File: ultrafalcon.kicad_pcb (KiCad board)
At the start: 2 copper layers, 66.3 x 66.3 mm, 1 part, among them SW1 RotaryEncoder

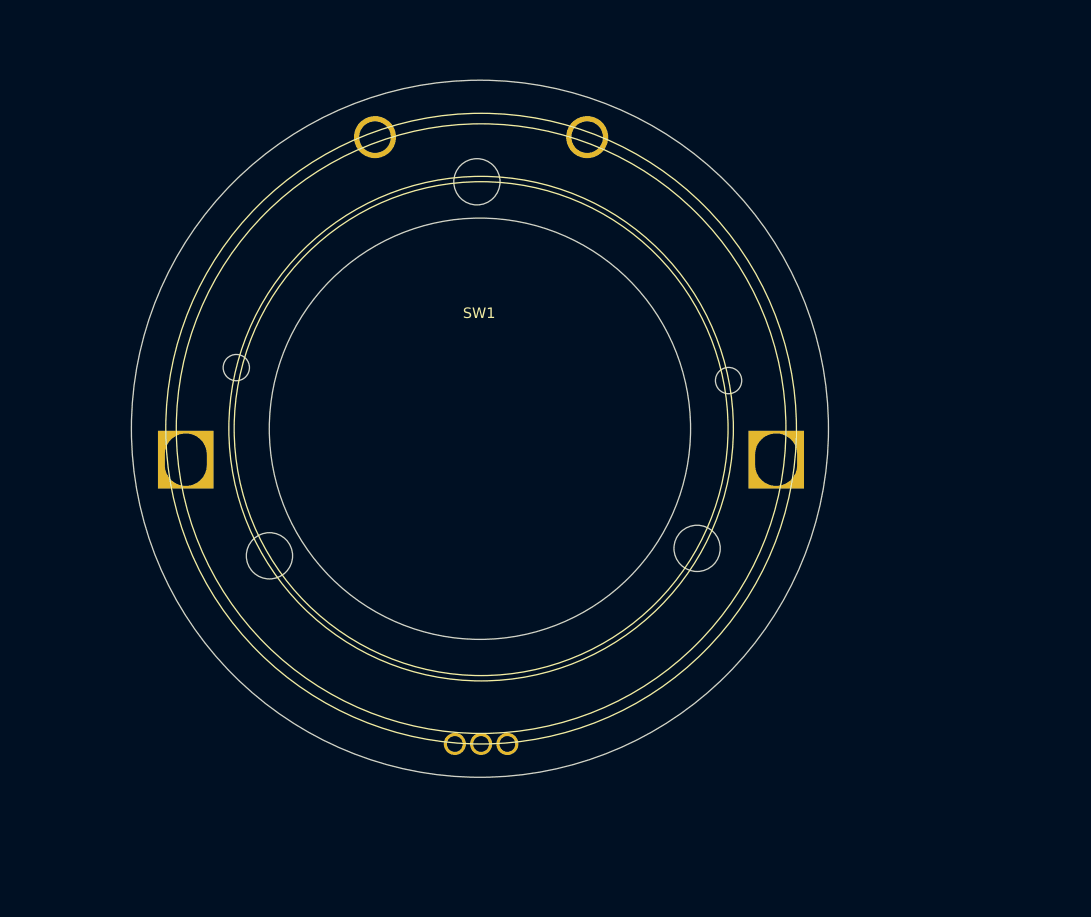
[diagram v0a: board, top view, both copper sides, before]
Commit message: jan17 updates
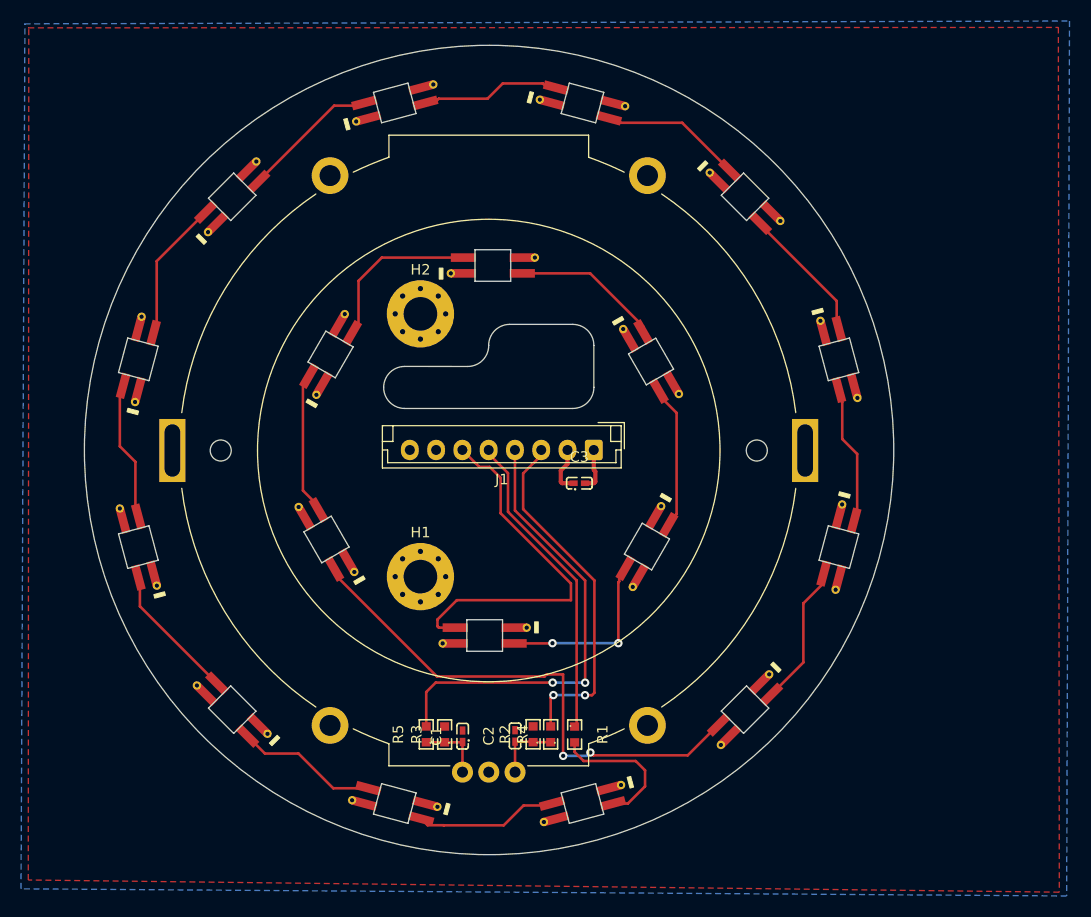
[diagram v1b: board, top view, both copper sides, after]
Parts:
- added C1: 0.01uF, ct-kicad:C0402, F.Cu at (147.5, 127.2)
- added C2: 0.01uF, ct-kicad:C0402, F.Cu at (152.5, 127.2)
- added C3: 1uF, ct-kicad:C0402, F.Cu at (158.6, 103.1)
- added H1: MountingHole, MountingHole:MountingHole_3.2mm_M3_Pad_Via, F.Cu at (143.5, 112.0)
- added H2: MountingHole, MountingHole:MountingHole_3.2mm_M3_Pad_Via, F.Cu at (143.5, 87.0)
- added J1: Conn_01x08_Socket, Connector_JST:JST_EH_B8B-EH-A_1x08_P2.50mm_Vertical, F.Cu at (160.0, 100.0)
- added R1: 330, ct-kicad:R0603, F.Cu at (158.2, 127.0)
- added R2: 10k, ct-kicad:R0603, F.Cu at (154.2, 127.0)
- added R3: 10k, ct-kicad:R0603, F.Cu at (145.8, 127.0)
- added R4: 10k, ct-kicad:R0603, F.Cu at (155.9, 127.0)
- added R5: 10k, ct-kicad:R0603, F.Cu at (144.1, 127.0)
- added U1: SK6812MINI-E_C5149201, ct-kicad:YS-SK6812MINI-E-casuanoob, F.Cu at (141.1, 66.9)
- added U10: SK6812MINI-E_C5149201, ct-kicad:YS-SK6812MINI-E-casuanoob, F.Cu at (116.7, 109.2)
- added U11: SK6812MINI-E_C5149201, ct-kicad:YS-SK6812MINI-E-casuanoob, F.Cu at (116.7, 91.3)
- added U12: SK6812MINI-E_C5149201, ct-kicad:YS-SK6812MINI-E-casuanoob, F.Cu at (125.6, 75.9)
- added U13: SK6812MINI-E_C5149201, ct-kicad:YS-SK6812MINI-E-casuanoob, F.Cu at (134.6, 108.5)
- added U14: SK6812MINI-E_C5149201, ct-kicad:YS-SK6812MINI-E-casuanoob, F.Cu at (134.9, 90.9)
- added U15: SK6812MINI-E_C5149201, ct-kicad:YS-SK6812MINI-E-casuanoob, F.Cu at (150.4, 82.4)
- added U16: SK6812MINI-E_C5149201, ct-kicad:YS-SK6812MINI-E-casuanoob, F.Cu at (165.4, 91.5)
- added U17: SK6812MINI-E_C5149201, ct-kicad:YS-SK6812MINI-E-casuanoob, F.Cu at (165.1, 109.1)
- added U18: SK6812MINI-E_C5149201, ct-kicad:YS-SK6812MINI-E-casuanoob, F.Cu at (149.6, 117.6)
- added U2: SK6812MINI-E_C5149201, ct-kicad:YS-SK6812MINI-E-casuanoob, F.Cu at (158.9, 66.9)
- added U3: SK6812MINI-E_C5149201, ct-kicad:YS-SK6812MINI-E-casuanoob, F.Cu at (174.4, 75.9)
- added U4: SK6812MINI-E_C5149201, ct-kicad:YS-SK6812MINI-E-casuanoob, F.Cu at (183.3, 91.3)
- added U5: SK6812MINI-E_C5149201, ct-kicad:YS-SK6812MINI-E-casuanoob, F.Cu at (183.3, 109.2)
- added U6: SK6812MINI-E_C5149201, ct-kicad:YS-SK6812MINI-E-casuanoob, F.Cu at (174.4, 124.7)
- added U7: SK6812MINI-E_C5149201, ct-kicad:YS-SK6812MINI-E-casuanoob, F.Cu at (158.9, 133.6)
- added U8: SK6812MINI-E_C5149201, ct-kicad:YS-SK6812MINI-E-casuanoob, F.Cu at (141.1, 133.6)
- added U9: SK6812MINI-E_C5149201, ct-kicad:YS-SK6812MINI-E-casuanoob, F.Cu at (125.6, 124.7)
- SW1: footprint fingerpunch:PERS56v3 -> ct-kicad:PER60
- moved SW1 2.20 mm to (150.0, 100.0)
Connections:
- SW1 pad A: unconnected-(SW1-PadA) -> Net-(C2-Pad1)
- SW1 pad B: unconnected-(SW1-PadB) -> Net-(C1-Pad1)
- SW1 pad C: unconnected-(SW1-PadC) -> GND
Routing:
- net Net-(U13-DIN): track 0.00 -> 50.5 mm, vias 0 -> 2
- net ENCODER_B: track 0.00 -> 43.7 mm, vias 0 -> 2
- net LED_DO: track 0.00 -> 35.0 mm
- net ENCODER_A: track 0.00 -> 33.7 mm, vias 0 -> 2
- net LED_DI: track 0.00 -> 29.9 mm
- net Net-(U17-DOUT): track 0.00 -> 17.3 mm, vias 0 -> 2
- net Net-(U14-DOUT): track 0.00 -> 16.1 mm
- net Net-(U1-DOUT): track 0.00 -> 14.3 mm
- net Net-(U15-DOUT): track 0.00 -> 14.1 mm
- net Net-(U16-DOUT): track 0.00 -> 13.8 mm
- net Net-(U13-DOUT): track 0.00 -> 13.6 mm
- net Net-(U7-DIN): track 0.00 -> 13.6 mm
- net Net-(U11-DOUT): track 0.00 -> 13.6 mm
- net Net-(U2-DOUT): track 0.00 -> 13.6 mm
- net Net-(U5-DOUT): track 0.00 -> 13.6 mm
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- added copper zone on B.Cu, net GND
- added copper zone on F.Cu, net GND
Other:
- board size 66.3 x 66.3 mm -> 77 x 77 mm
